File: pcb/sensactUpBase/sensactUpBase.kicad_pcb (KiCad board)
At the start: 2 copper layers, 50 x 50 mm, 8 parts, among them J1 BaseConnect, J10 24 GN CH CL 24 GN CH CL, J3 T2 T1 T1, J4 B RS485 A, J9 T3 T4 T5 T6 T7 GN 3V GN SC SD, U1 PCA9555PW

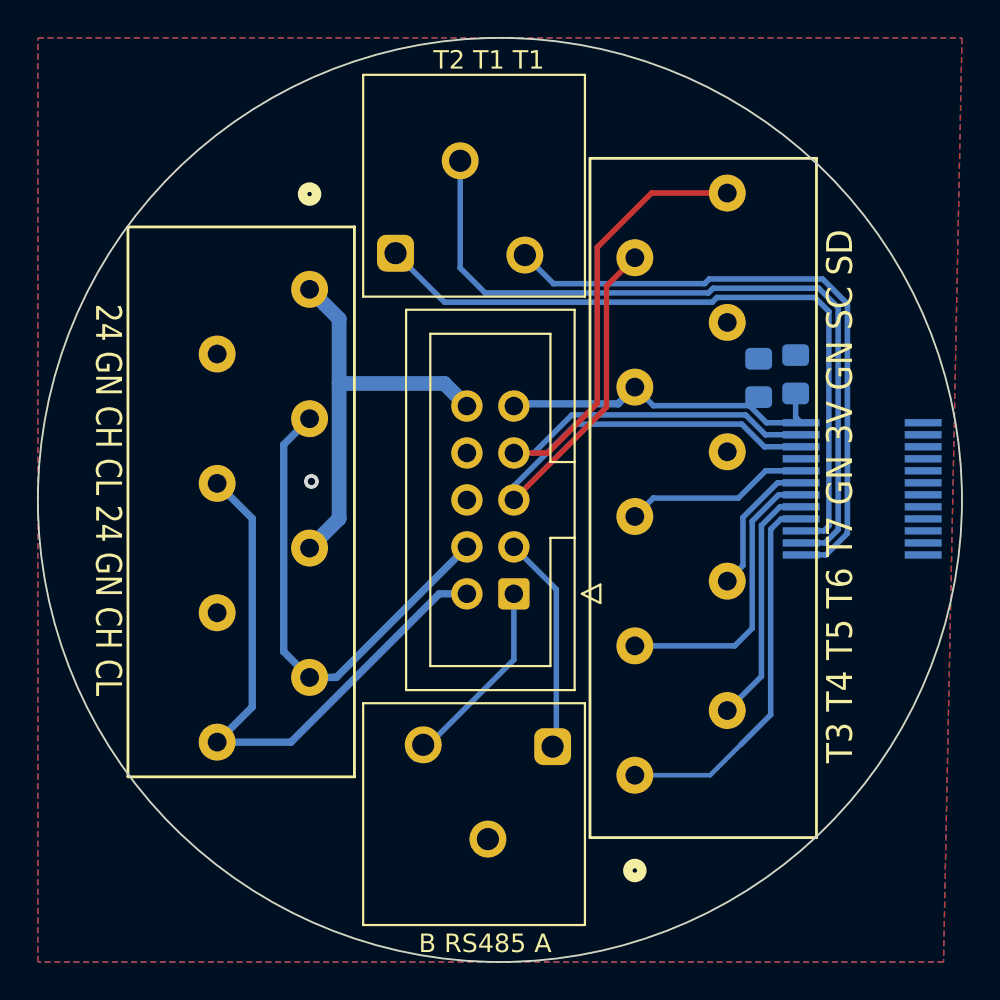
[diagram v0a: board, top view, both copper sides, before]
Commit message: Updated various PCB
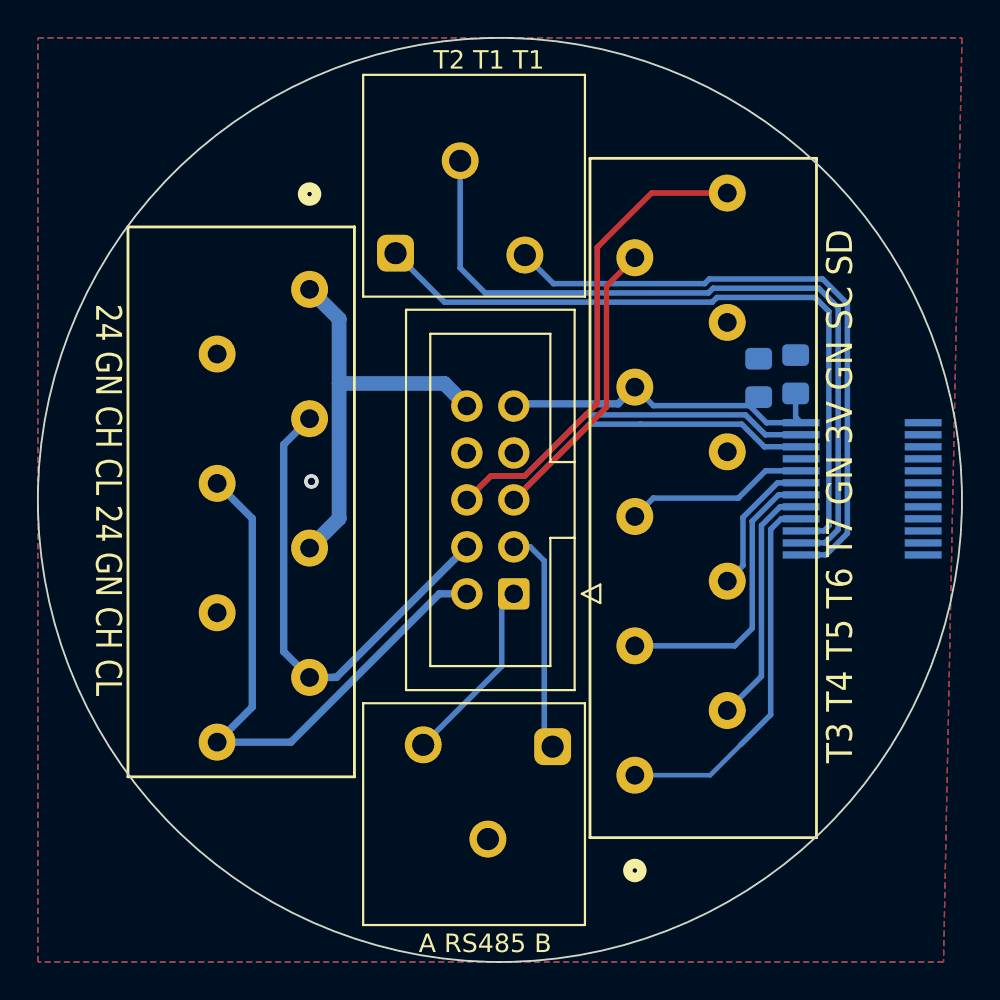
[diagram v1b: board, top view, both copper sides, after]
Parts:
- J4: value B RS485 A -> A RS485 B
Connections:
- J1 pad 1: RS485B -> RS485A
- J1 pad 3: RS485A -> RS485B
- J1 pad 6: GND -> SDA
- J1 pad 7: SDA -> GND
- J4 pad 1: RS485A -> RS485B
- J4 pad 3: RS485B -> RS485A
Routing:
- net SDA: track 38.8 -> 46.0 mm
- net RS485A: track 11.8 -> 10.2 mm
